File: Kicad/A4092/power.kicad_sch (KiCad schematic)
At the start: 35 parts, among them J7 22112042

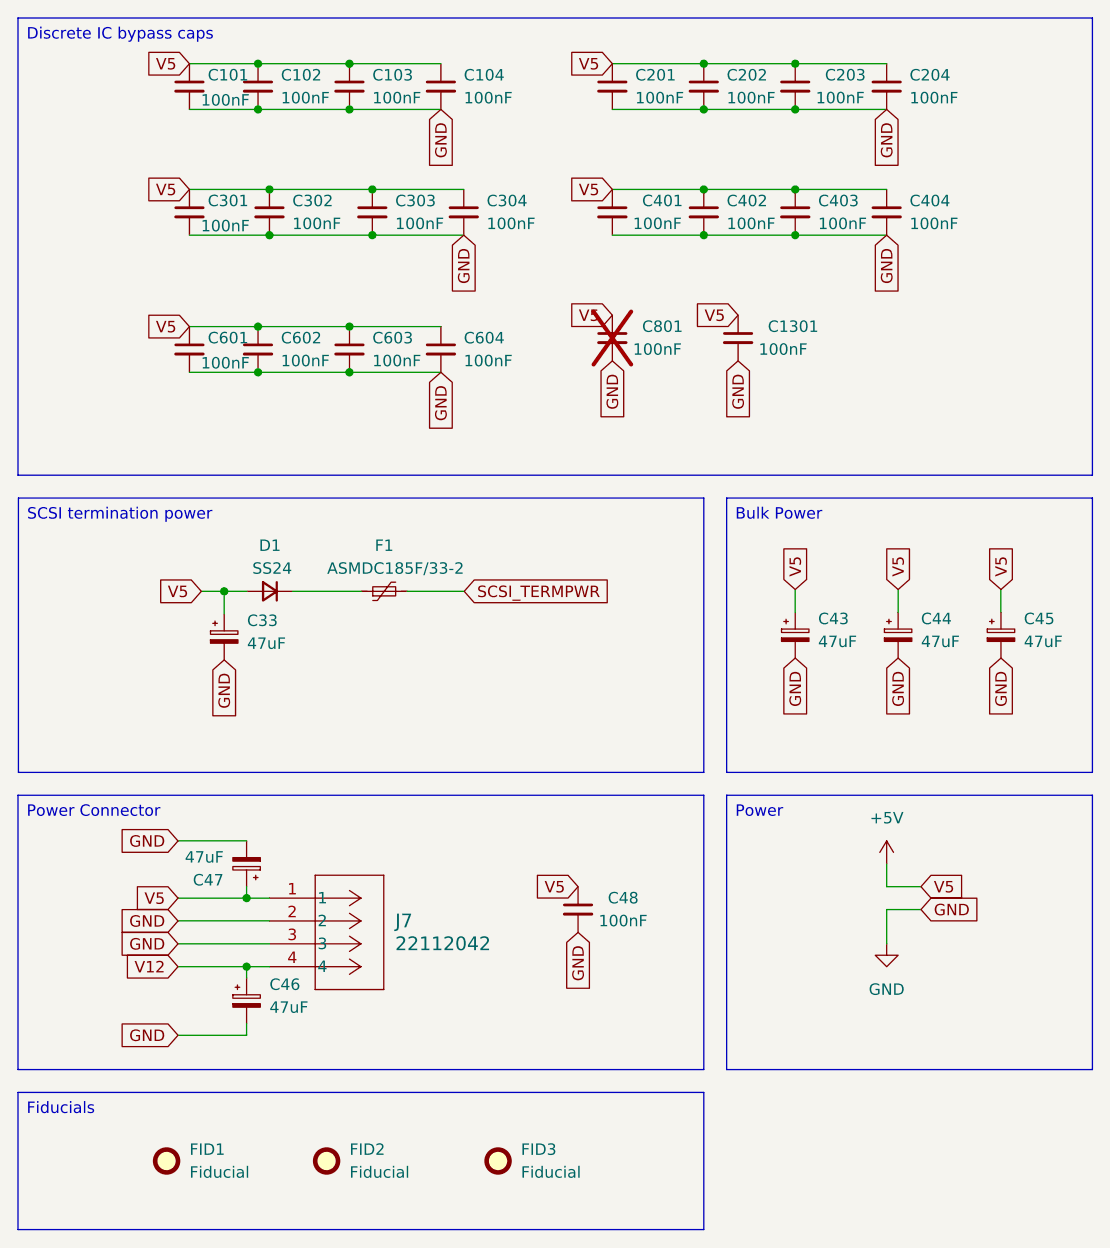
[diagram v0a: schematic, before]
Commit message: First version of A4770 cheetah
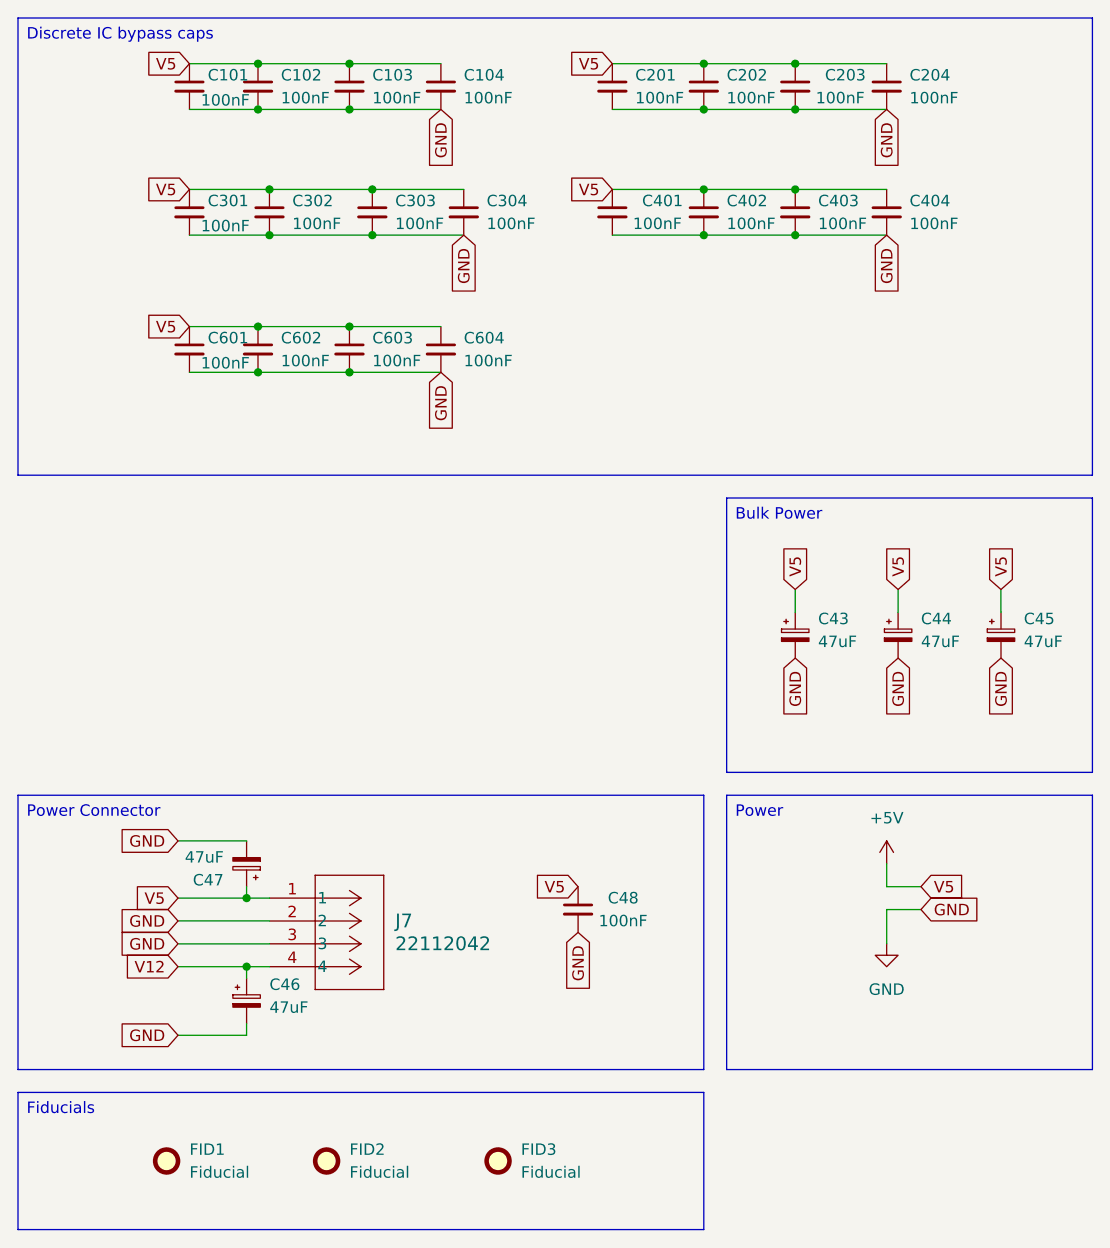
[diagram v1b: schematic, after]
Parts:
- removed C1301, C801: 100nF, Capacitor_SMD:C_0603_1608Metric_Pad1.08x0.95mm_HandSolder, symbol Device:C_Small
- removed C33: 47uF, Capacitor_SMD:CP_Elec_6.3x7.7, symbol Device:C_Polarized_Small
- removed D1: SS24, Diode_SMD:D_SMA_Handsoldering, symbol Device:D_Small
- removed F1: ASMDC185F/33-2, Fuse:Fuse_2920_7451Metric_Pad2.10x5.45mm_HandSolder, symbol Device:Polyfuse_Small
